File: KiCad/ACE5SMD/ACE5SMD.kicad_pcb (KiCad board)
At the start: 2 copper layers, 160 x 100 mm, 94 parts, among them IC1 LM7805_TO220, Q1 MMBT3904, Q3 BC847, X1 CRYSTALHC49U-V 6.556MHz, X2 5MHz

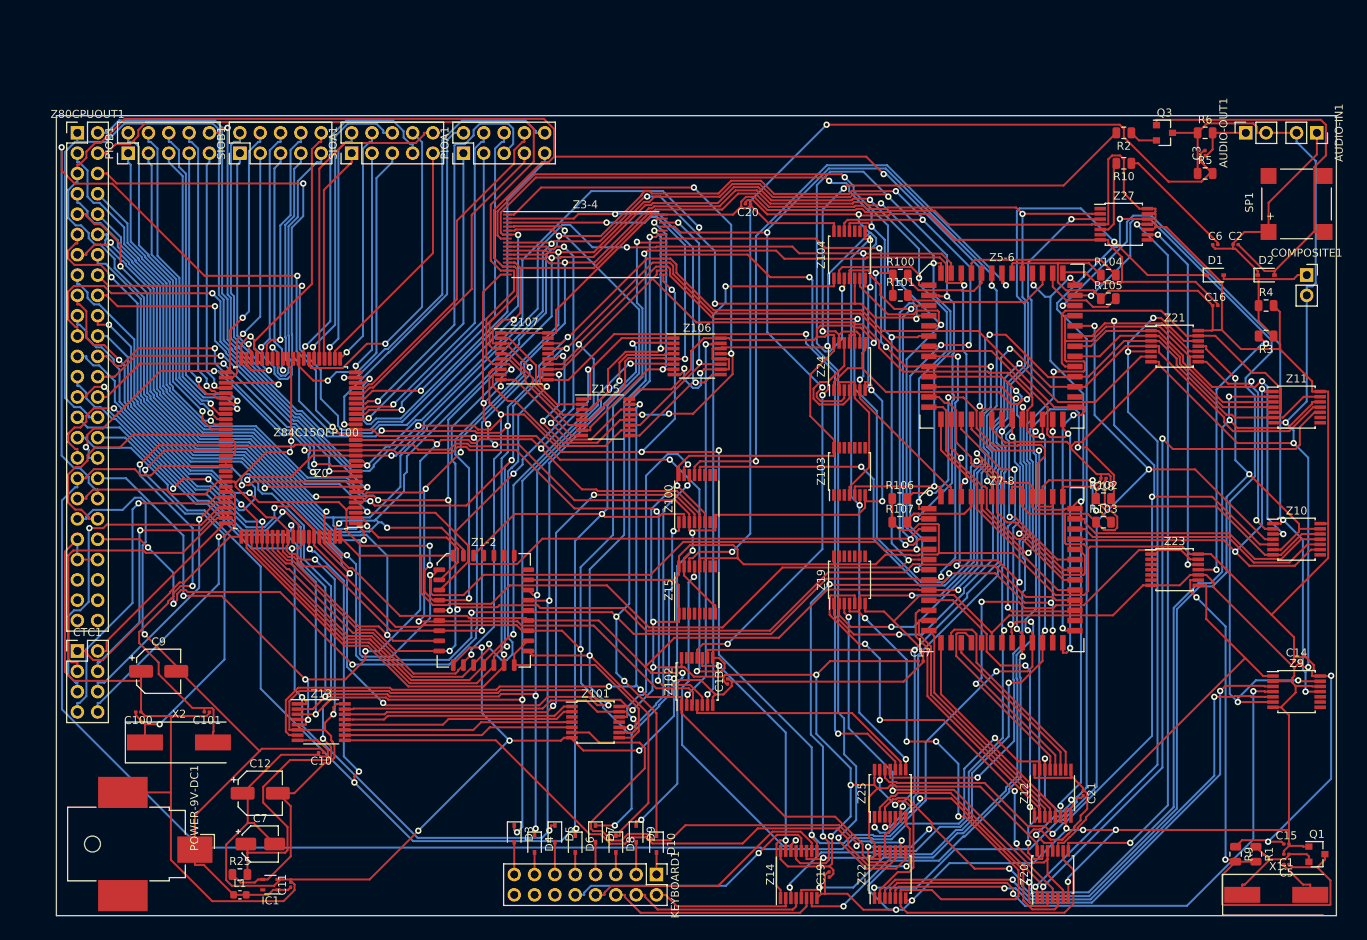
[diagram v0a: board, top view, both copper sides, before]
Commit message: UPdate to latest version.
Signed-off-by: John Bradley <flypie@rocketmail.com>
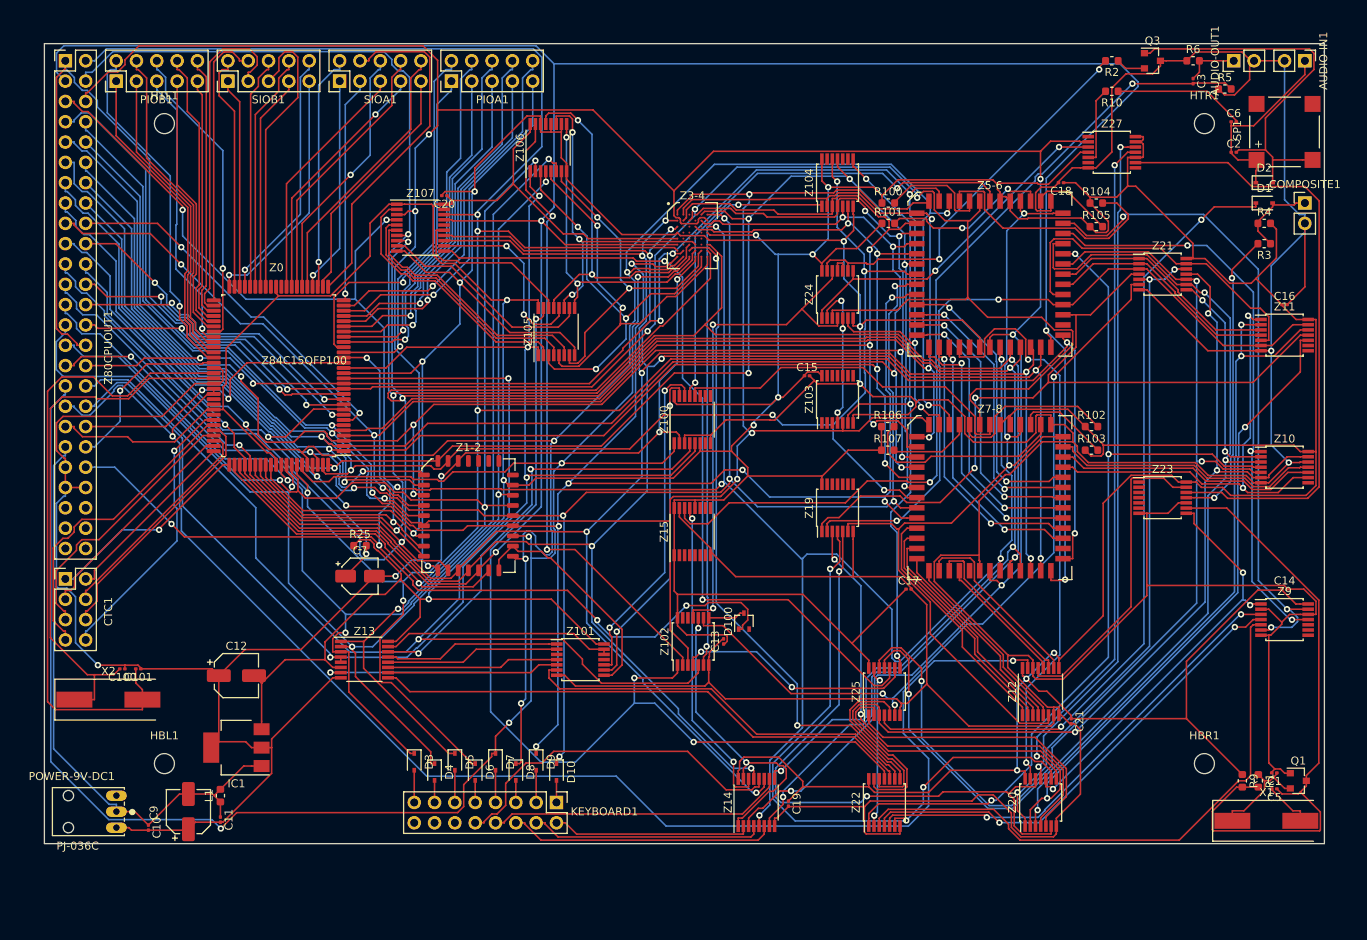
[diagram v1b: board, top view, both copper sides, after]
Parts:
- added D100: BAT54W, Package_TO_SOT_SMD:SOT-323_SC-70, F.Cu at (154.4, 118.2)
- added HBL1: MountingHole, MountingHole:MountingHole_2.5mm, F.Cu at (82.0, 136.0)
- added HBR1: MountingHole, MountingHole:MountingHole_2.5mm, F.Cu at (212.0, 136.0)
- added HTL1: MountingHole, MountingHole:MountingHole_2.5mm, F.Cu at (82.0, 56.0)
- added HTR1: MountingHole, MountingHole:MountingHole_2.5mm, F.Cu at (212.0, 56.0)
- AUDIO-IN1, AUDIO-OUT1, COMPOSITE1: footprint Connector_PinSocket_2.54mm:PinSocket_1x02_P2.54mm_Vertical -> Connector_PinHeader_2.54mm:PinHeader_1x02_P2.54mm_Vertical
- IC1: footprint Package_TO_SOT_SMD:SOT-343_SC-70-4 -> Package_TO_SOT_SMD:SOT-223-3_TabPin2
- L1: value L -> 100 nH
- POWER-9V-DC1: value Conn_01x02 -> PJ-036C; footprint Connector_BarrelJack:BarrelJack_CUI_PJ-036AH-SMT_Horizontal -> cuipj:CUI_PJ-036C
- R1, R10, R100, R101, R102, R103, R104, R105, R106, R107, R2, R25, R3, R4, R5, R6, R9: footprint Resistor_SMD:R_0805_2012Metric -> Resistor_SMD:R_0603_1608Metric
- Z3-4: footprint Package_SO:TSOP-I-32_18.4x8mm_P0.5mm -> Package_BGA:FBGA-48_6x8_6.0x8.0mm
- moved C15 83.8 mm to (162.3, 87.5)
- moved R25 43.8 mm to (106.4, 108.8)
- moved C20 38.0 mm to (117.0, 65.0)
- moved C18 37.3 mm to (194.1, 63.4)
- moved C7 35.7 mm to (106.4, 112.6)
- moved Z106 32.0 mm to (130.0, 59.0), turned to 90 degrees
- moved C10 23.5 mm to (80.0, 144.0), turned to 270 degrees
- moved Z107 20.7 mm to (114.0, 69.0)
- moved C9 17.9 mm to (85.0, 142.0), turned to 90 degrees
- moved IC1 17.6 mm to (91.0, 134.0)
- moved C6 15.5 mm to (215.7, 55.8)
- moved D10 15.4 mm to (131.0, 137.0)
- moved D4 15.4 mm to (115.8, 137.0)
- moved D8 15.4 mm to (125.9, 137.0)
- moved KEYBOARD1 15.4 mm to (131.0, 140.9)
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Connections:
- POWER-9V-DC1 pad 3: (no net) -> Net-(POWER-9V-DC1-Pad3)
- Z102 pad 8: //INT -> Net-(D100-Pad3)
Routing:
- net /A6: track 283.4 -> 196.1 mm
- net /A12: track 247.3 -> 163.0 mm
- net /A5: track 278.0 -> 204.3 mm, vias 5 -> 6
- net //HALT: track 108.3 -> 37.7 mm, vias 3 -> 2
- net /A2: track 271.3 -> 202.9 mm, vias 10 -> 6
- net /DA6: track 283.1 -> 349.8 mm, vias 6 -> 4
- net /DA1: track 375.9 -> 310.1 mm, vias 7 -> 9
- net /A7: track 253.2 -> 188.8 mm, vias 9 -> 5
- net #RESET: track 114.6 -> 69.5 mm
- net /A11: track 201.3 -> 244.4 mm, vias 6 -> 5
- net //IOREQ: track 115.6 -> 157.4 mm, vias 5 -> 2
- net +5V: track 887.7 -> 848.7 mm, vias 15 -> 11
- net /A8: track 272.2 -> 237.8 mm
- net //INT: track 159.6 -> 125.6 mm, vias 6 -> 5
- net GND: track 998.2 -> 965.2 mm, vias 30 -> 11
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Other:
- net class Default: trace_width 0.25 -> 0.2
- net class SMD added: clearance 0.1524, trace_width 0.2, via_dia 0.8, via_drill 0.4
